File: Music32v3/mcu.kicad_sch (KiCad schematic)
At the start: 6 parts, among them SW1 SW_Push, U1 ESP32-WROOM-32E__16MB_

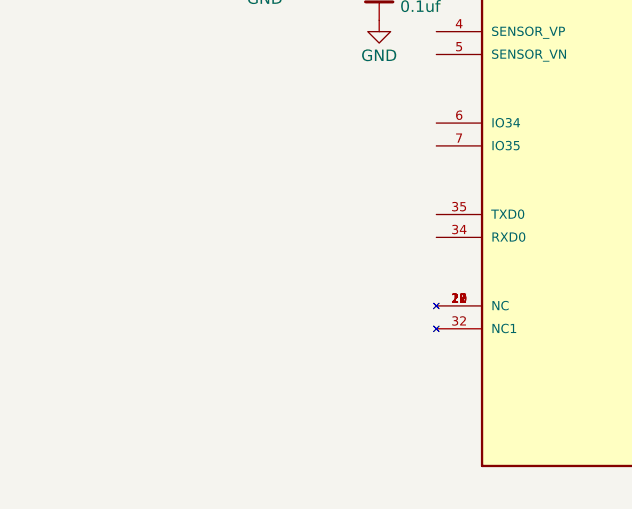
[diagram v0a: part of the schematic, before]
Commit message: SD card and usb and power
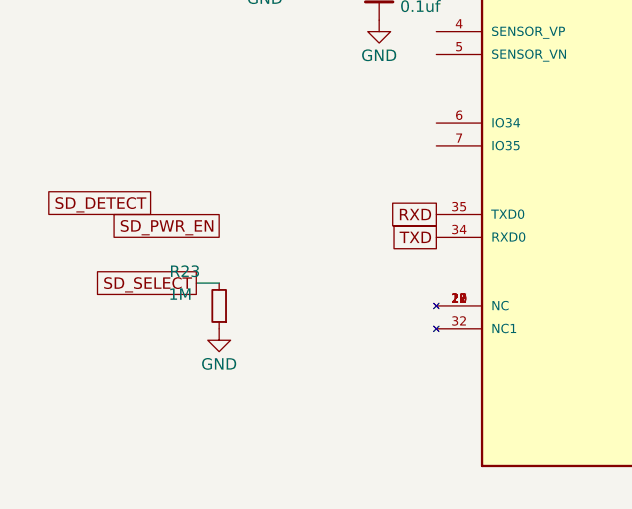
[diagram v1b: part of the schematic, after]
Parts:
- added R23: 1M, Resistor_SMD:R_0402_1005Metric, symbol Device:R_Small
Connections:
- net GND: now also R23.1
- net TXD: now reaches U1.34 (RXD0)
- net RXD: now reaches U1.35 (TXD0)
- new net SD_SELECT: R23.2
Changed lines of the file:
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@@
+    (stroke (width 0) (type default))
+  )
+  (wire (pts (xy 97.79 106.68) (xy 95.25 106.68))
     (stroke (width 0) (type default))
   )
@@
     (stroke (width 0) (type default))
   )
+  (global_label "TXD" (shape passive) (at 121.92 101.6 180) (fields_autoplaced)
+    (effects (font (size 1.27 1.27)) (justify right))
+    (property "Intersheetrefs" "${INTERSHEET_REFS}" (at 116.6784 101.6 0)
+      (effects (font (size 1.27 1.27)) (justify right) hide)
+    )
+  )
+  (global_label "SD_DETECT" (shape passive) (at 90.17 97.79 180) (fields_autoplaced)
+    (effects (font (size 1.27 1.27)) (justify right))
+    (property "Intersheetrefs" "${INTERSHEET_REFS}" (at 78.1552 97.79 0)
+      (effects (font (size 1.27 1.27)) (justify right) hide)
+    )
+  )
+  (global_label "SD_SELECT" (shape passive) (at 95.25 106.68 180) (fields_autoplaced)
+    (effects (font (size 1.27 1.27)) (justify right))
+    (property "Intersheetrefs" "${INTERSHEET_REFS}" (at 83.2352 106.68 0)
+      (effects (font (size 1.27 1.27)) (justify right) hide)
+    )
+  )
+  (global_label "SD_PWR_EN" (shape passive) (at 97.79 100.33 180) (fields_autoplaced)
+    (effects (font (size 1.27 1.27)) (justify right))
+    (property "Intersheetrefs" "${INTERSHEET_REFS}" (at 85.1099 100.33 0)
+      (effects (font (size 1.27 1.27)) (justify right) hide)
+    )
+  )
+  (global_label "RXD" (shape passive) (at 121.92 99.06 180) (fields_autoplaced)
+    (effects (font (size 1.27 1.27)) (justify right))
+    (property "Intersheetrefs" "${INTERSHEET_REFS}" (at 116.376 99.06 0)
+      (effects (font (size 1.27 1.27)) (justify right) hide)
+    )
+  )
   (symbol (lib_id "Switch:SW_Push") (at 107.95 71.12 0) (unit 1)
     (in_bom yes) (on_board yes) (dnp no) (fields_autoplaced)
@@
     )
   )
+  (symbol (lib_id "Device:R_Small") (at 97.79 109.22 180) (unit 1)
+    (in_bom yes) (on_board yes) (dnp no)
+    (property "Reference" "R23" (at 93.98 105.41 0)
+      (effects (font (size 1.27 1.27)))
+    )
+    (property "Value" "1M" (at 93.472 107.95 0)
+      (effects (font (size 1.27 1.27)))
+    )
+    (property "Footprint" "Resistor_SMD:R_0402_1005Metric" (at 97.79 109.22 0)
+      (effects (font (size 1.27 1.27)) hide)
+    )
+    (property "Datasheet" "~" (at 97.79 109.22 0)
+      (effects (font (size 1.27 1.27)) hide)
+    )
+    (property "MPN_LCSC" "1" (at 97.79 109.22 90)
+      (effects (font (size 1.27 1.27)) hide)
+    )
+    (property "Price_LCSC" "0.0005" (at 97.79 109.22 90)
+      (effects (font (size 1.27 1.27)) hide)
+    )
+    (pin "1")
+    (pin "2")
+    (instances
+      (project "Power"
+        (path "/1288f273-4ee1-44e8-a86c-2adc0358dc71"
+          (reference "R23") (unit 1)
+        )
+      )
+      (project "Music_32_V2"
+        (path "/14681cc8-ddd4-43ff-b571-daca84d76d6b/4963a591-4c7d-4c5c-bcea-2e6cea395856"
+          (reference "R23") (unit 1)
+        )
+        (path "/14681cc8-ddd4-43ff-b571-daca84d76d6b/386f7fcb-de3c-43a3-99bd-dcf77f99c217"
+          (reference "R31") (unit 1)
+        )
+      )
+      (project "Music32v3"
+        (path "/492e826b-8900-4c12-8604-1c812b2e1995"
+          (reference "R13") (unit 1)
+        )
+        (path "/492e826b-8900-4c12-8604-1c812b2e1995/4998783d-7055-40b0-9979-647930a37834"
+          (reference "R13") (unit 1)
+        )
+        (path "/492e826b-8900-4c12-8604-1c812b2e1995/3c978059-9f1a-4ff6-9071-c1971133aa54"
+          (reference "R14") (unit 1)
+        )
+        (path "/492e826b-8900-4c12-8604-1c812b2e1995/af454206-d75b-4aff-be43-99164678694a"
+          (reference "R15") (unit 1)
+        )
+      )
+      (project "Phone"
+        (path "/9a44bf40-ccf4-4ff9-bb89-c8bc2c0cf19f/08dec41e-a7ac-46dd-ad42-4ddeee026110/46f942c4-bdd7-445d-bd75-6b4493769f4c"
+          (reference "R?") (unit 1)
+        )
+      )
+      (project "Ipod"
+        (path "/c4cf9ad0-abea-4c32-bb0b-367e5261d002"
+          (reference "R?") (unit 1)
+        )
+        (path "/c4cf9ad0-abea-4c32-bb0b-367e5261d002/683020cc-3f85-458f-8fb0-f668196e1562"
+          (reference "R22") (unit 1)
+        )
+      )
+      (project "power"
+        (path "/c90b3fe4-1e97-415b-a0f6-be34dcca7903"
+          (reference "R?") (unit 1)
+        )
+      )
+      (project "Power"
+        (path "/e4f8ce38-95ca-4021-bdd0-de4735b761e8"
+          (reference "R?") (unit 1)
+        )
+      )
+    )
+  )
   (symbol (lib_id "power:GND") (at 162.56 124.46 0) (unit 1)
     (in_bom yes) (on_board yes) (dnp no) (fields_autoplaced)
@@
         )
       )
+    )
+  )
+  (symbol (lib_id "power:GND") (at 97.79 111.76 0) (unit 1)
+    (in_bom yes) (on_board yes) (dnp no) (fields_autoplaced)
+    (property "Reference" "#PWR076" (at 97.79 118.11 0)
+      (effects (font (size 1.27 1.27)) hide)
+    )
+    (property "Value" "GND" (at 97.79 115.705 0)
+      (effects (font (size 1.27 1.27)))
+    )
+    (property "Footprint" "" (at 97.79 111.76 0)
+      (effects (font (size 1.27 1.27)) hide)
+    )
+    (property "Datasheet" "" (at 97.79 111.76 0)
+      (effects (font (size 1.27 1.27)) hide)
+    )
+    (pin "1")
+    (instances
+      (project "Music32v3"
+        (path "/492e826b-8900-4c12-8604-1c812b2e1995/af454206-d75b-4aff-be43-99164678694a"
+          (reference "#PWR076") (unit 1)
+        )
+      )

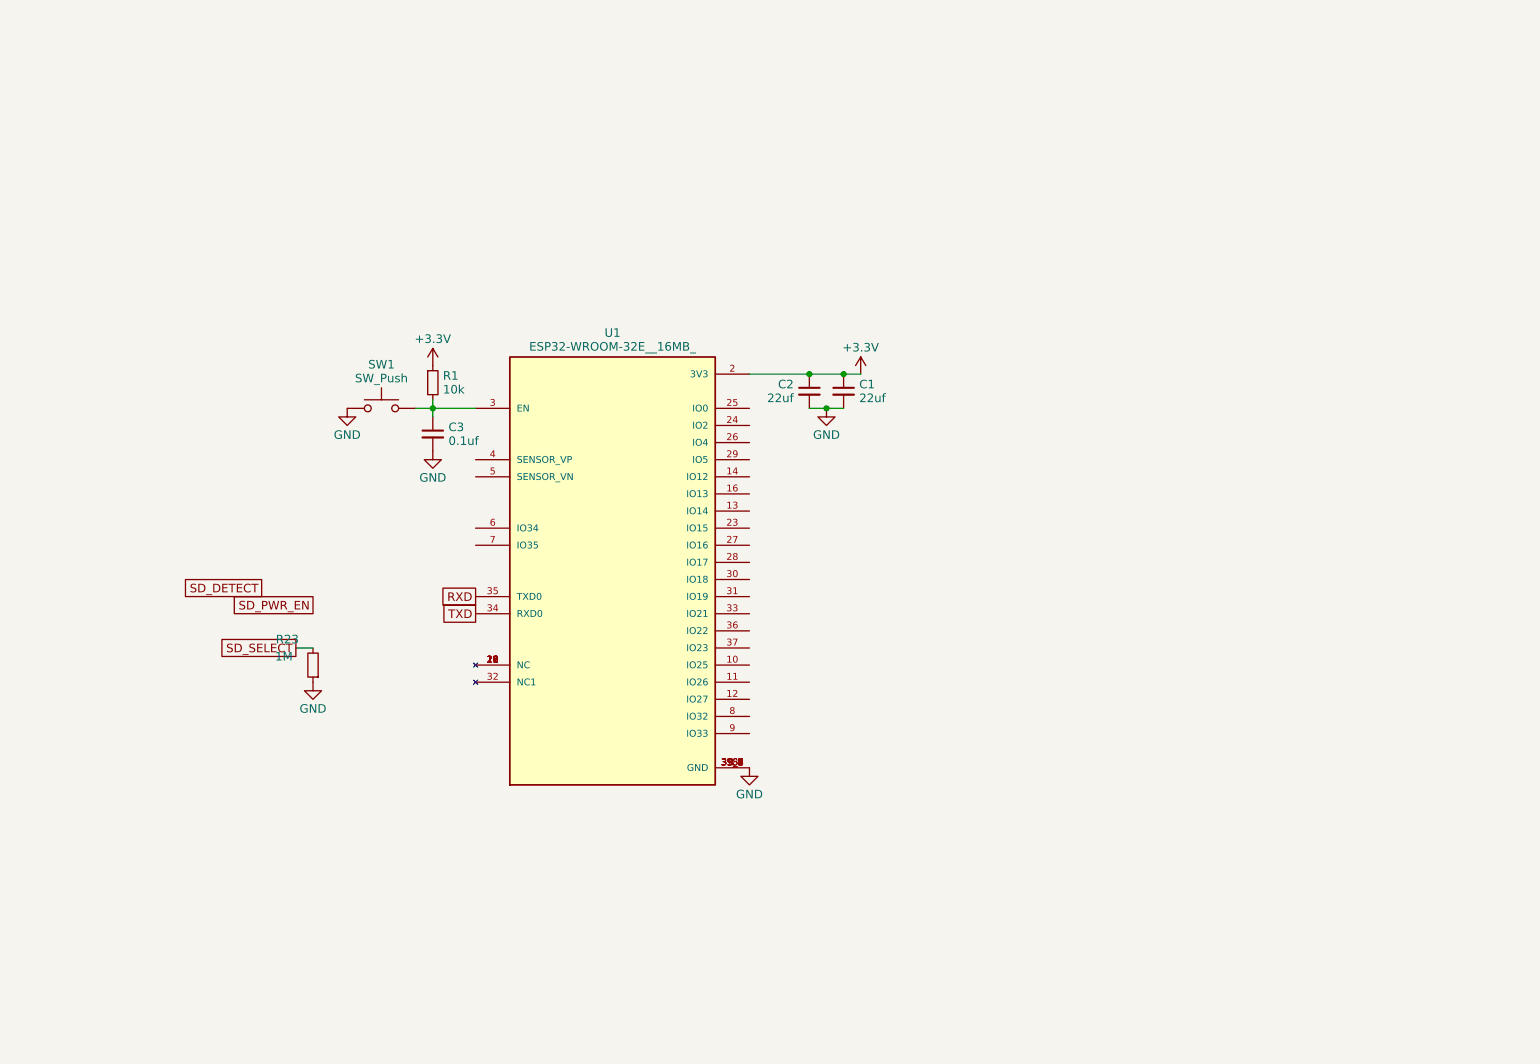
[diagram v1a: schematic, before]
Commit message: Schematic
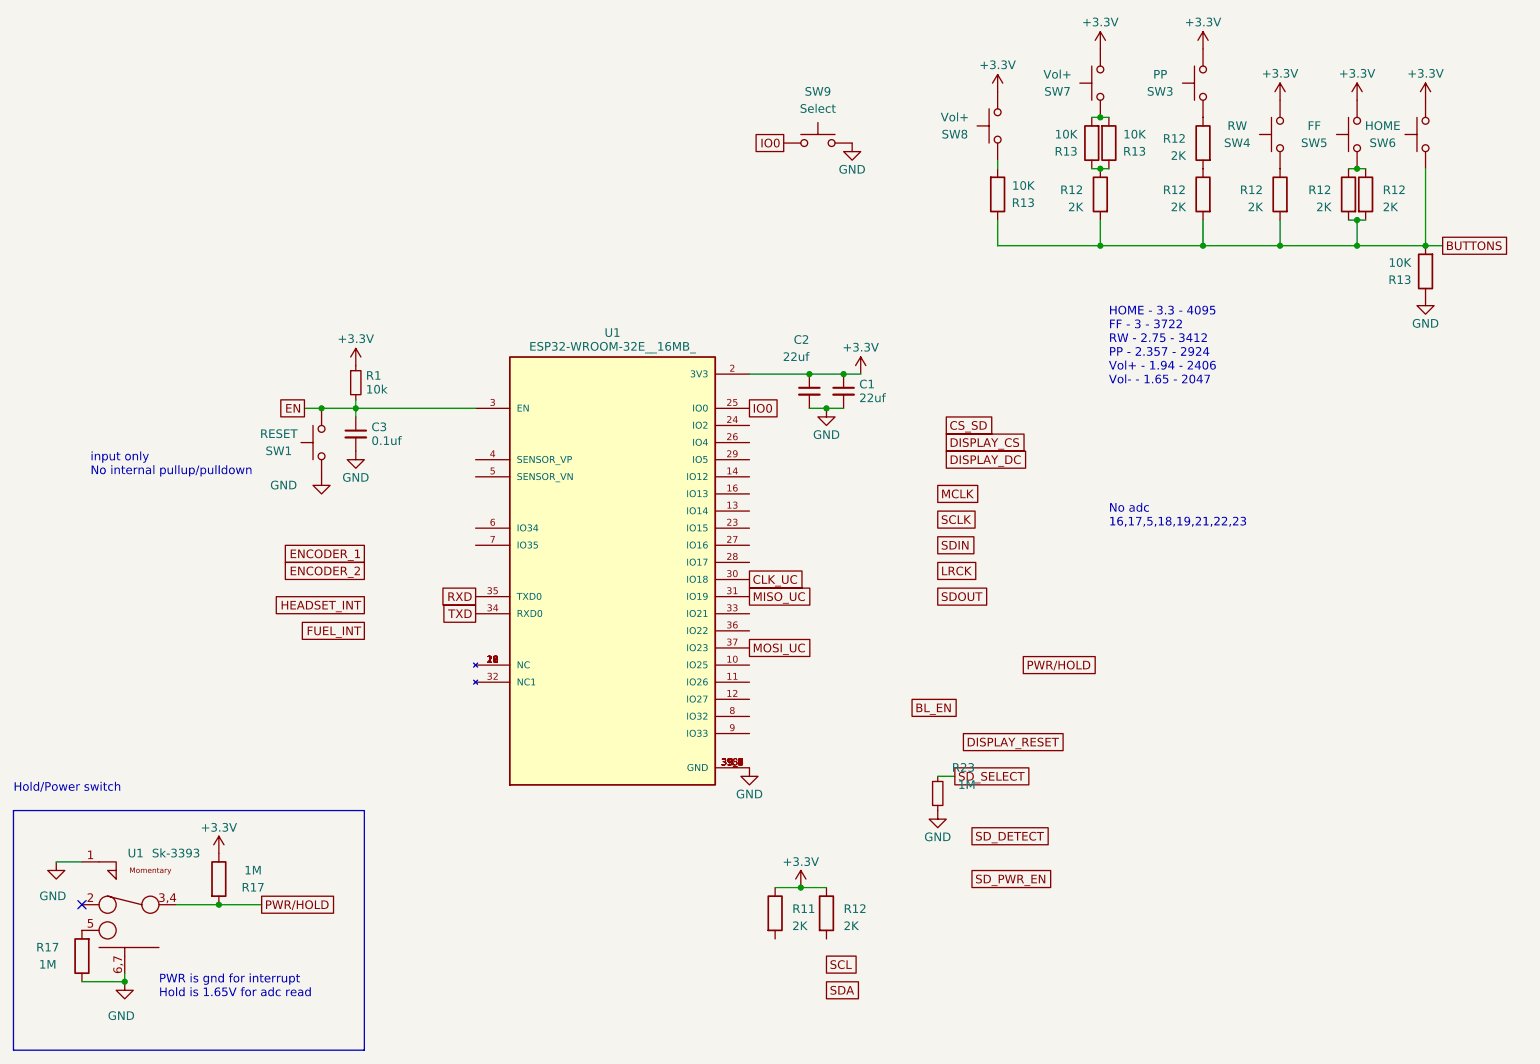
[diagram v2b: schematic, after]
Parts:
- added R11, R12 (x7): 2K, Resistor_SMD:R_0402_1005Metric, symbol Device:R
- added R13 (x4): 10K, Resistor_SMD:R_0402_1005Metric, symbol Device:R
- added R17 (x2): 1M, Resistor_SMD:R_0402_1005Metric, symbol Device:R
- added SW3: PP, Music:TS3315A, symbol Switch:SW_Push
- added SW4: RW, Music:TS3315A, symbol Switch:SW_Push
- added SW5: FF, Music:TS3315A, symbol Switch:SW_Push
- added SW6: HOME, Music:TS3315A, symbol Switch:SW_Push
- added SW7, SW8: Vol+, Music:TSA002A3816B04, symbol Switch:SW_Push
- added SW9: Select, Music:TS3315A, symbol Switch:SW_Push
- added U1: Sk-3393, Music:SK-3393M-G1, symbol sk-3393m-g1:_SK-3393M-G1
- C1, C2: footprint (none) -> Capacitor_SMD:C_0805_2012Metric
- C3: footprint (none) -> Capacitor_SMD:C_0402_1005Metric
- R1: footprint (none) -> Resistor_SMD:R_0402_1005Metric
- SW1: value SW_Push -> RESET; footprint (none) -> Music:TS3315A
- U1: footprint ESP32-WROOM-32E__16MB_:XCVR_ESP32-WROOM-32E__16MB_ -> Music:ESP32-WROOM-32E
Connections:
- net +3.3V: now also R11.1, R12.1, R17.1, SW3.2, SW4.2, SW5.2, SW6.2, SW7.2, SW8.2
- net GND: now also R13.1, R17.1, SW9.2, U1.1, U1.6,7
- net EN: now reaches C3.1, R1.2, SW1.2, U1.3 (EN)
- net IO0: now reaches U1.25 (IO0)
- net IO0: now also SW9.1
- net CLK_UC: now reaches U1.30 (IO18)
- net MISO_UC: now reaches U1.31 (IO19)
- net MOSI_UC: now reaches U1.37 (IO23)
- new net: R12.1, SW4.1
- new net: R13.2, SW8.1
- new net: R12.1, R13.1, R13.1
- new net: R13.2, R13.2, SW7.1
- new net: R12.1, R12.1, SW5.1
- new net: R17.2, U1.5
- new net: R12.1, SW3.1
- new net: R12.1, R12.2
- new net BUTTONS: R12.2, R12.2, R12.2, R12.2, R12.2, R13.1, R13.2, SW6.1
- new net PWR/HOLD: R17.2, U1.3,4
- no-connect marks 0 -> 1
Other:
- note added: "HOME - 3.3 - 4095 FF - 3 - 3722 RW - 2.75 - 3412 PP - 2.357 - 2924 Vol+ - 1.94 - 2406 Vol- - 1.65 - 2047"
- note added: "Hold/Power switch"
- note added: "No adc 16,17,5,18,19,21,22,23"
- note added: "PWR is gnd for interrupt Hold is 1.65V for adc read"
- note added: "input only No internal pullup/pulldown"
- moved on the sheet: C3, R1, R23, SW1
